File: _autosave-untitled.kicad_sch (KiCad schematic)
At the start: 47 parts, among them J1 USB1, J2 USB1, J3 Conn_01x15_Pin, J4 Conn_01x15_Pin, SW1 SW_Push, SW3 SW_Push, U1 ESP32-S3, U2 W25Q16JVSS, U3 ME6231A33PG, U4 CH343P, Y1 Crystal_GND24, Y2 Crystal

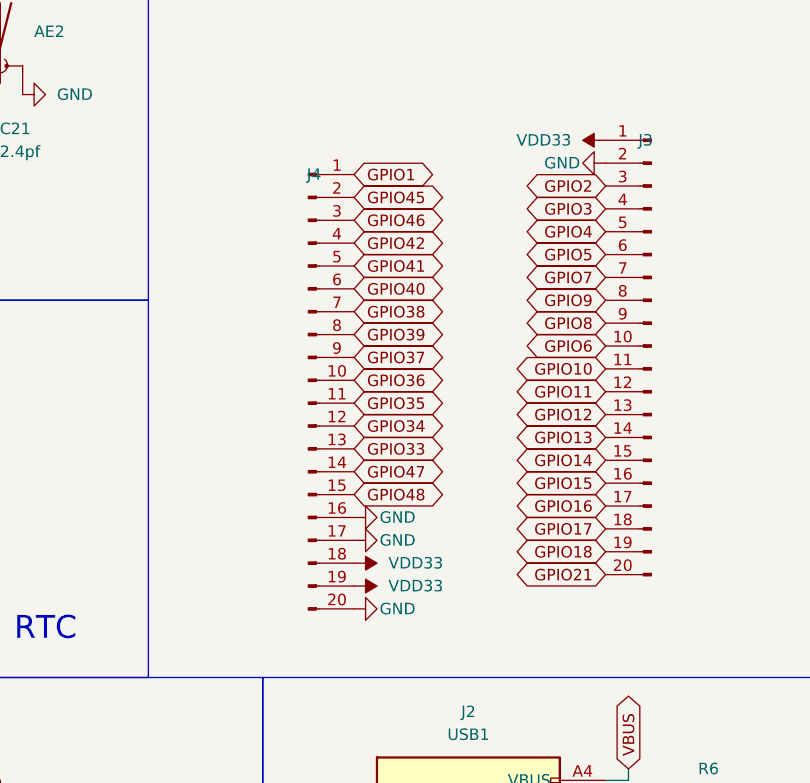
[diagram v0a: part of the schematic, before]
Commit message: 初步完成PCB
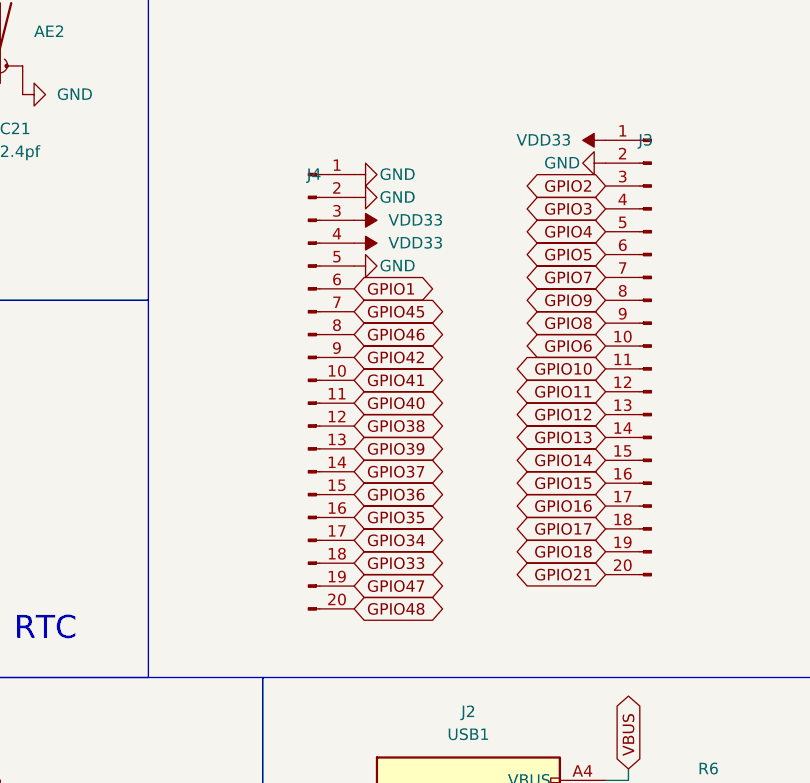
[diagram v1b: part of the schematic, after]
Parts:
- SW1, SW3: footprint SmartLock:SW-SMD_L3.9-W3.0-P4.45 -> smartlock:SW-SMD_L3.9-W3.0-P4.45
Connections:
- net GND: now also J4.1 (Pin_1), J4.2 (Pin_2), J4.5 (Pin_5); no longer J4.16 (Pin_16), J4.17 (Pin_17), J4.20 (Pin_20)
- net GPIO1: now also J4.6 (Pin_6); no longer J4.1 (Pin_1)
- net GPIO33: now also J4.18 (Pin_18); no longer J4.13 (Pin_13)
- net GPIO34: now also J4.17 (Pin_17); no longer J4.12 (Pin_12)
- net GPIO35: now also J4.16 (Pin_16); no longer J4.11 (Pin_11)
- net GPIO36: now also J4.15 (Pin_15); no longer J4.10 (Pin_10)
- net GPIO37: now also J4.14 (Pin_14); no longer J4.9 (Pin_9)
- net GPIO38: now also J4.12 (Pin_12); no longer J4.7 (Pin_7)
- net GPIO39: now also J4.13 (Pin_13); no longer J4.8 (Pin_8)
- net GPIO40: now also J4.11 (Pin_11); no longer J4.6 (Pin_6)
- net GPIO41: now also J4.10 (Pin_10); no longer J4.5 (Pin_5)
- net GPIO42: now also J4.9 (Pin_9); no longer J4.4 (Pin_4)
- net GPIO45: now also J4.7 (Pin_7); no longer J4.2 (Pin_2)
- net GPIO46: now also J4.8 (Pin_8); no longer J4.3 (Pin_3)
- net GPIO47: now also J4.19 (Pin_19); no longer J4.14 (Pin_14)
- net GPIO48: now also J4.20 (Pin_20); no longer J4.15 (Pin_15)
- net VDD33: now also J4.3 (Pin_3), J4.4 (Pin_4); no longer J4.18 (Pin_18), J4.19 (Pin_19)
